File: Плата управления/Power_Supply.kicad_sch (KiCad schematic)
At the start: 24 parts, among them U3 LMV321

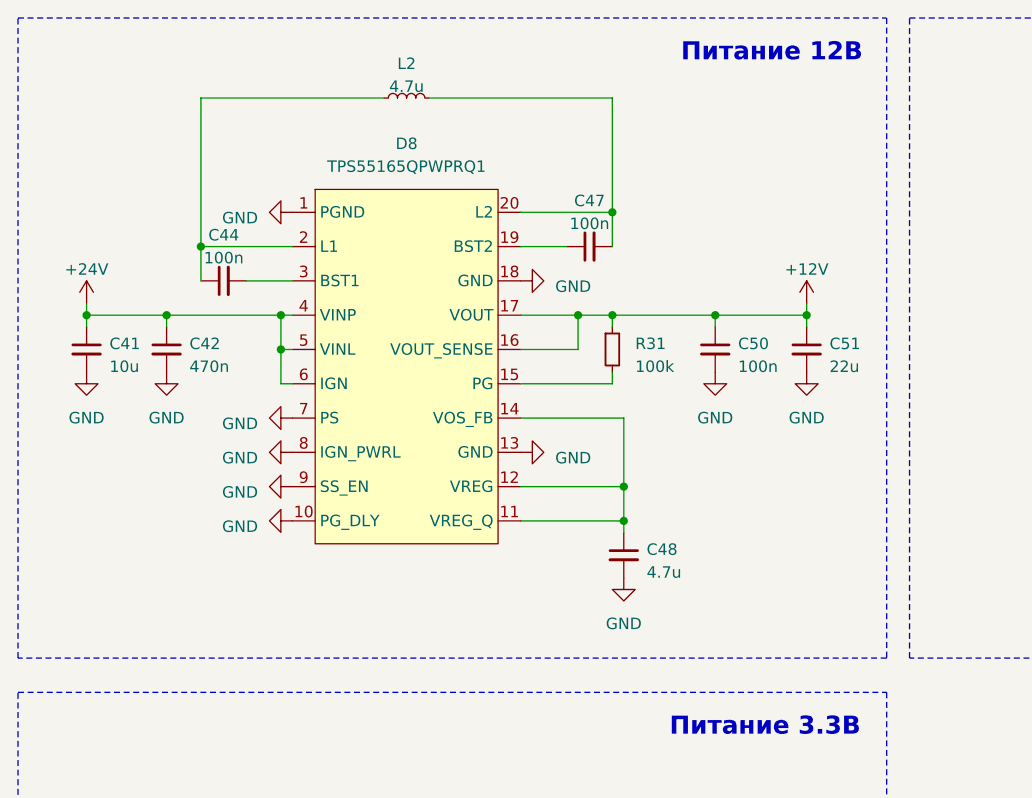
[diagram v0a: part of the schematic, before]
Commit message: Ещё нужно доработать
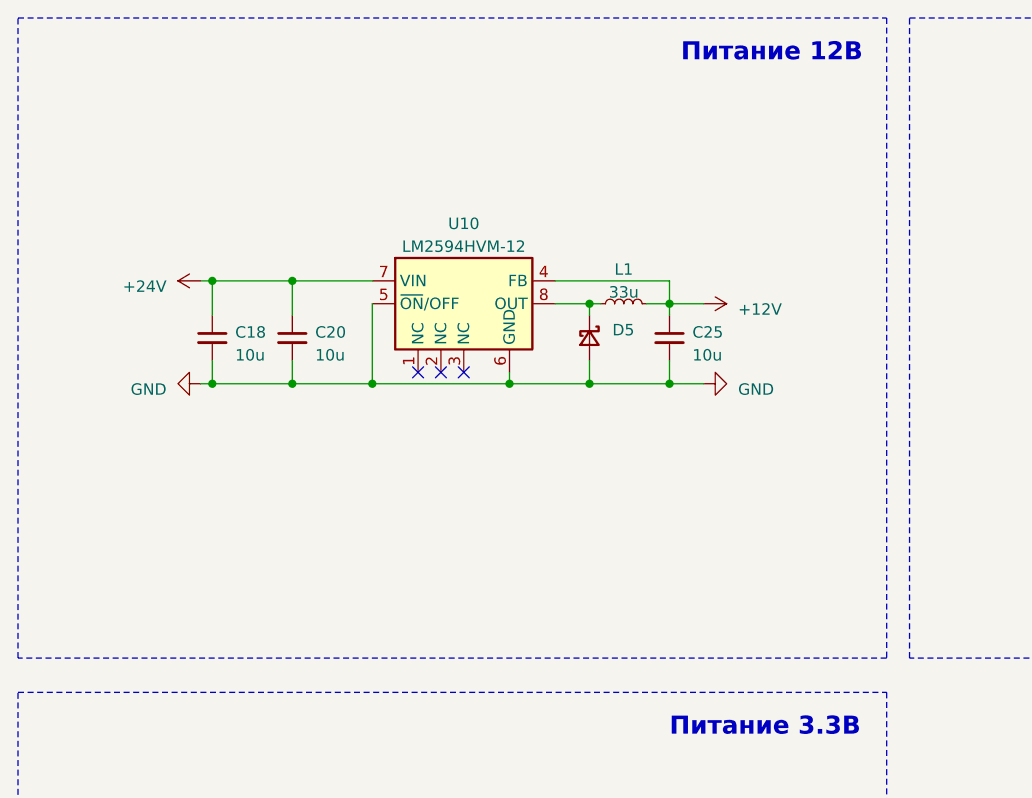
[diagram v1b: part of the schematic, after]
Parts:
- removed C41: 10u, Capacitor_SMD:C_1210_3225Metric_Pad1.33x2.70mm_HandSolder, symbol Device:C_Small
- removed C42: 470n, Capacitor_SMD:C_0805_2012Metric_Pad1.18x1.45mm_HandSolder, symbol Device:C_Small
- removed C44, C47, C50: 100n, Capacitor_SMD:C_0603_1608Metric_Pad1.08x0.95mm_HandSolder, symbol Device:C_Small
- removed C48: 4.7u, Capacitor_SMD:C_0805_2012Metric_Pad1.18x1.45mm_HandSolder, symbol Device:C_Small
- removed C51: 22u, Capacitor_SMD:C_1210_3225Metric_Pad1.33x2.70mm_HandSolder, symbol Device:C_Small
- removed D8: TPS55165QPWPRQ1, Package_SO:HTSSOP-20-1EP_4.4x6.5mm_P0.65mm_EP3.4x6.5mm, symbol Connverter_DCDC_My:TPS55165QPWPRQ1
- removed L2: 4.7u, Inductor_my:LQH66SN100M03L, symbol Device:L_Small
- removed R31: 100k, Resistor_SMD:R_0603_1608Metric_Pad0.98x0.95mm_HandSolder, symbol Device:R_Small
- added C18, C20, C25: 10u, Capacitor_SMD:C_1210_3225Metric_Pad1.33x2.70mm_HandSolder, symbol Device:C_Small
- added D5: MBRA320, Diode_SMD:D_SMA, symbol Device:D_Schottky_Small
- added L1: 33u, Inductor_SMD:L_10.4x10.4_H4.8, symbol Device:L_Small
- added U10: LM2594HVM-12, Package_SO:SOIC-8_3.9x4.9mm_P1.27mm, symbol Regulator_Switching:LM2594HVM-12
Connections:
- net +12V: now also C25.1, L1.2, U10.4 (FB)
- net +24V: now also C18.1, C20.1, U10.7 (VIN)
- net GND: now also C18.2, C20.2, C25.2, D5.2 (A), U10.5 (~{ON}/OFF), U10.6 (GND)
- new net: D5.1 (K), L1.1, U10.8 (OUT)
- no-connect marks 2 -> 5
